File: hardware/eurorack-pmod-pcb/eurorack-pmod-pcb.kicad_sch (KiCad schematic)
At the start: 2 parts

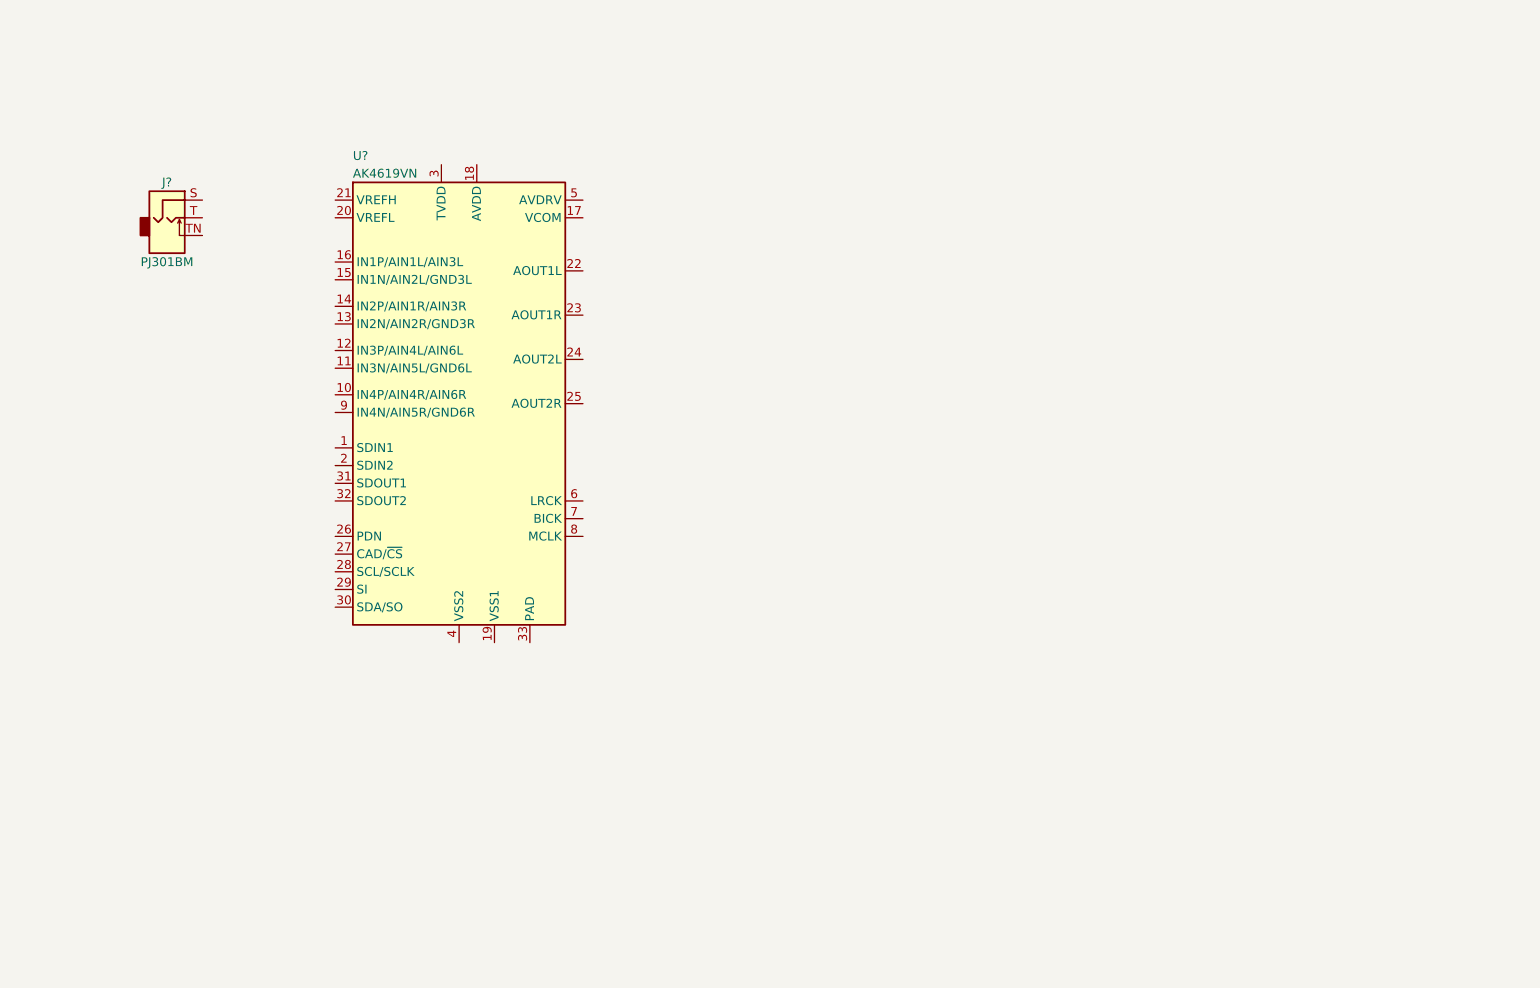
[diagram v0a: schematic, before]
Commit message: Finish schematic with AK4619, need to decide on other features
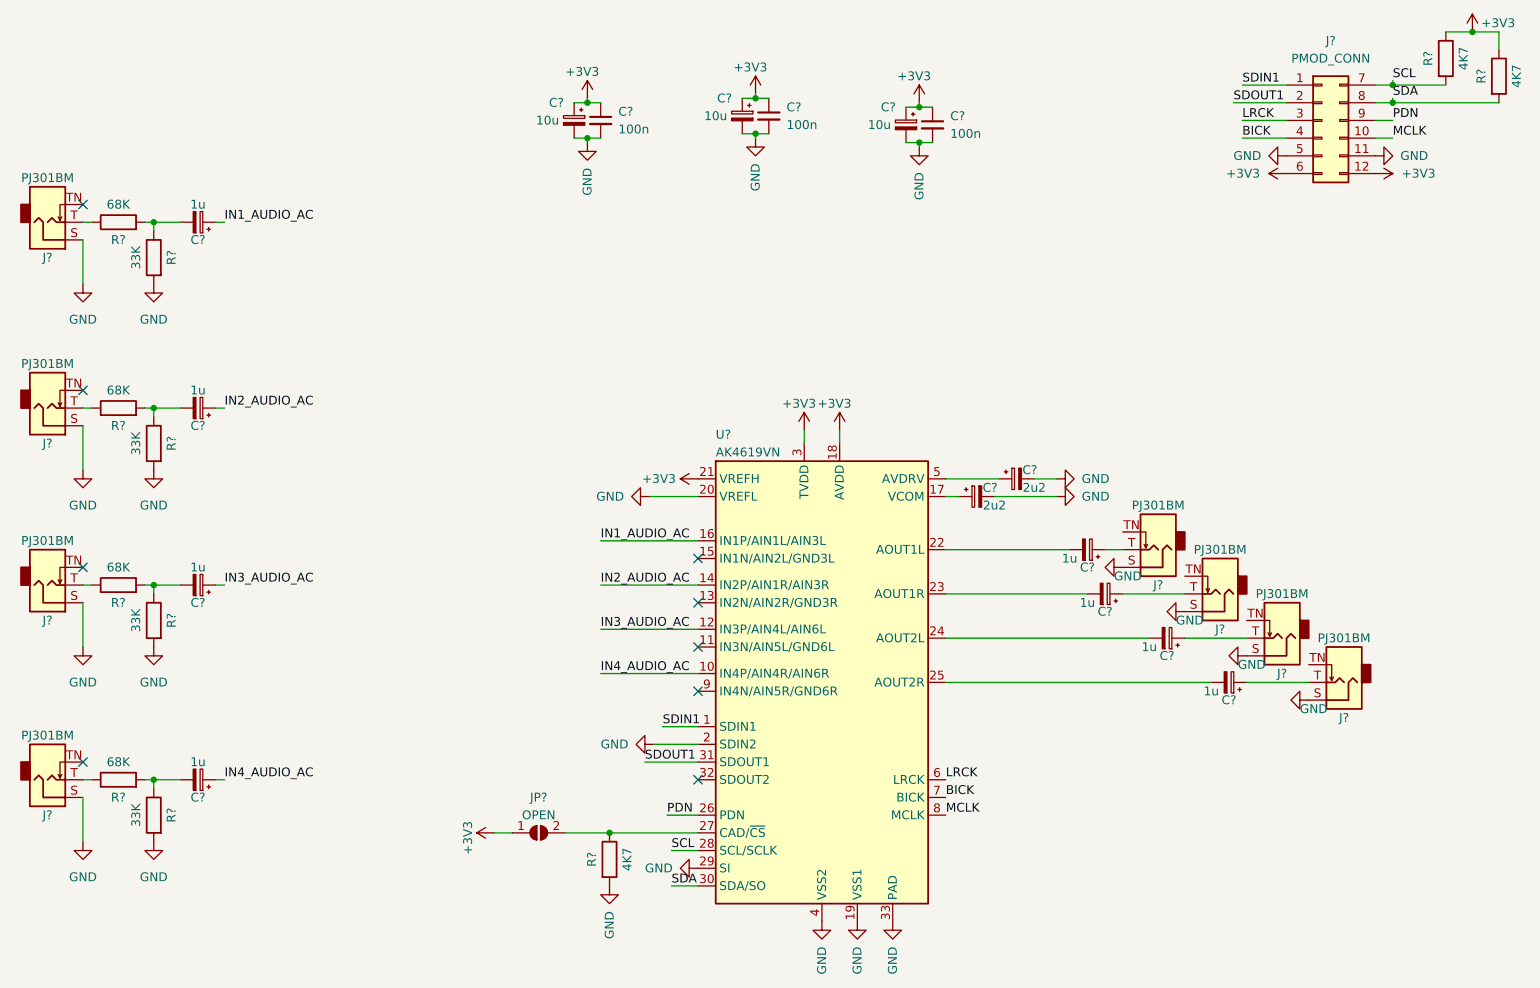
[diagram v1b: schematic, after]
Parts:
- added C? (x2): 2u2, symbol Device:C_Polarized_Small
- added C? (x3): 10u, symbol Device:C_Polarized_Small
- added C? (x8): 1u, symbol Device:C_Polarized_Small
- added C? (x3): 100n, symbol Device:C_Small
- added J? (x7): PJ301BM, AudioJacks:Jack_3.5mm_QingPu_WQP-PJ301BM_Vertical, symbol Connector:AudioJack2_SwitchT
- added J?: PMOD_CONN, symbol Connector_Generic:Conn_02x06_Top_Bottom
- added JP?: OPEN, symbol Jumper:SolderJumper_2_Open
- added R? (x4): 33K, symbol Device:R
- added R? (x4): 68K, symbol Device:R
- added R? (x3): 4K7, symbol Device:R
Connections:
- net GND: now reaches J?.S
- net GND: now also U?.19 (VSS1), U?.2 (SDIN2), U?.20 (VREFL), U?.29 (SI), U?.33 (PAD), U?.4 (VSS2), C?.2, C?.2, C?.2, C?.2, C?.2, C?.2, C?.2, C?.2, J?.11 (Pin_11), J?.5 (Pin_5), J?.S, J?.S, J?.S, J?.S, J?.S, J?.S, J?.S, R?.2, R?.2, R?.2, R?.2, R?.2
- net at J?.T: now also R?.1
- net SDIN1: now reaches U?.1 (SDIN1)
- net SDIN1: now also J?.1 (Pin_1)
- net IN4_AUDIO_AC: now reaches U?.10 (IN4P/AIN4R/AIN6R)
- net IN4_AUDIO_AC: now also C?.1
- net IN3_AUDIO_AC: now reaches U?.12 (IN3P/AIN4L/AIN6L)
- net IN3_AUDIO_AC: now also C?.1
- net IN2_AUDIO_AC: now reaches U?.14 (IN2P/AIN1R/AIN3R)
- net IN2_AUDIO_AC: now also C?.1
- net IN1_AUDIO_AC: now reaches U?.16 (IN1P/AIN1L/AIN3L)
- net IN1_AUDIO_AC: now also C?.1
- net at U?.17 (VCOM): now also C?.1
- net +3V3: now reaches U?.18 (AVDD)
- net +3V3: now also U?.21 (VREFH), U?.3 (TVDD), C?.1, C?.1, C?.1, C?.1, C?.1, C?.1, J?.12 (Pin_12), J?.6 (Pin_6), JP?.1 (A), R?.1, R?.1
- net at U?.22 (AOUT1L): now also C?.2
- net at U?.23 (AOUT1R): now also C?.2
- net at U?.24 (AOUT2L): now also C?.2
- net at U?.25 (AOUT2R): now also C?.2
- net PDN: now reaches U?.26 (PDN)
- net PDN: now also J?.9 (Pin_9)
- net at U?.27 (CAD/~{CS}): now also JP?.2 (B), R?.1
- net SCL: now reaches U?.28 (SCL/SCLK)
- net SCL: now also J?.7 (Pin_7), R?.2
- net SDA: now reaches U?.30 (SDA/SO)
- net SDA: now also J?.8 (Pin_8), R?.2
- net SDOUT1: now reaches U?.31 (SDOUT1)
- net SDOUT1: now also J?.2 (Pin_2)
- net at U?.5 (AVDRV): now also C?.1
- net LRCK: now reaches U?.6 (LRCK)
- net LRCK: now also J?.3 (Pin_3)
- net BICK: now reaches U?.7 (BICK)
- net BICK: now also J?.4 (Pin_4)
- net MCLK: now reaches U?.8 (MCLK)
- net MCLK: now also J?.10 (Pin_10)
- new net: J?.T, R?.1 (x3)
- new net: C?.2, R?.1, R?.2 (x4)
- new net: C?.1, J?.T (x4)
- no-connect marks 0 -> 9
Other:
- moved on the sheet: J?, U?
